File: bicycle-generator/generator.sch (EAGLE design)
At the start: 78 parts, among them IC1 MC34063AD, IC2 MC34063SO, K1 ARK500/2, K2 ARK500/2, K3 ARK500/2, K4 ARK500/2, K5 ARK500/2, K6 HEAT_NPN, K7 ARK500/2, K8 ARK500/2, Q1 IRF3704S, Q2 IRF740, Q3 MPSA56, Q4 IRF740, Q5 MPSA56, T1 BC807, T2 BC807, X1 CV_LED, X2 PWR_LED, X3 5V_SW, X4 5V_LED, X5 5V_OUT

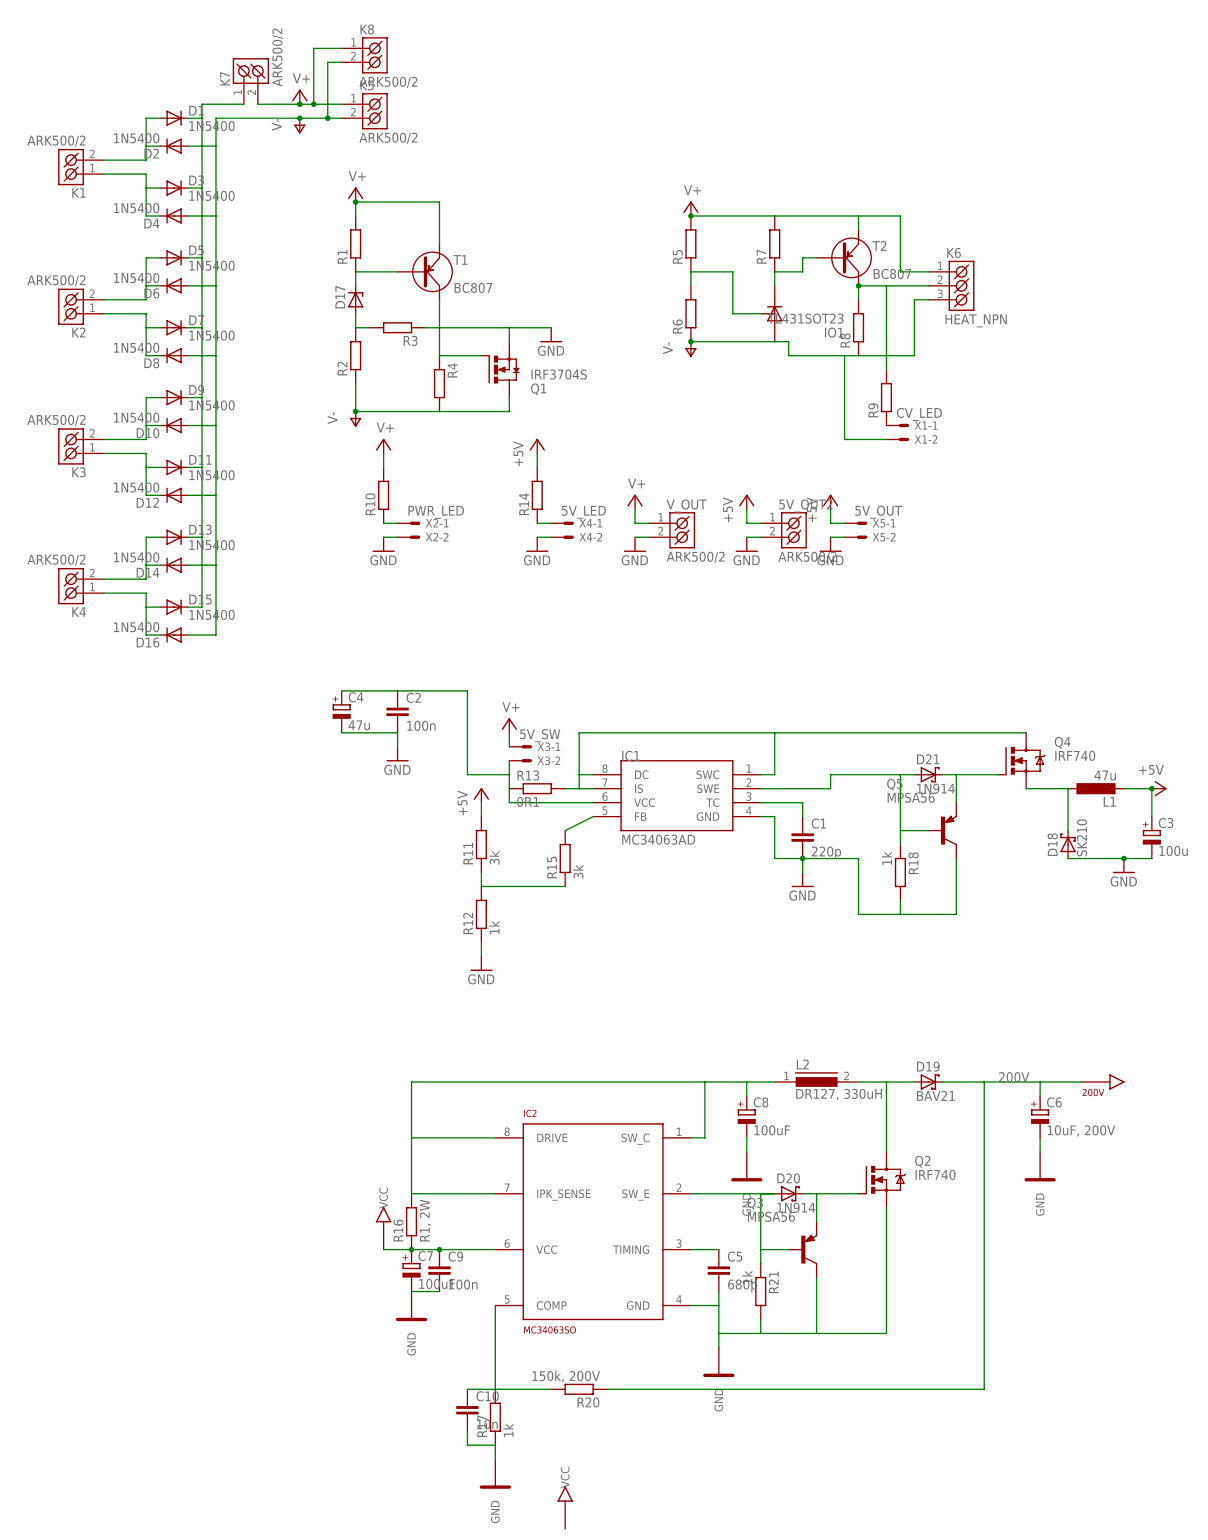
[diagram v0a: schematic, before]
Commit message: First version routed.
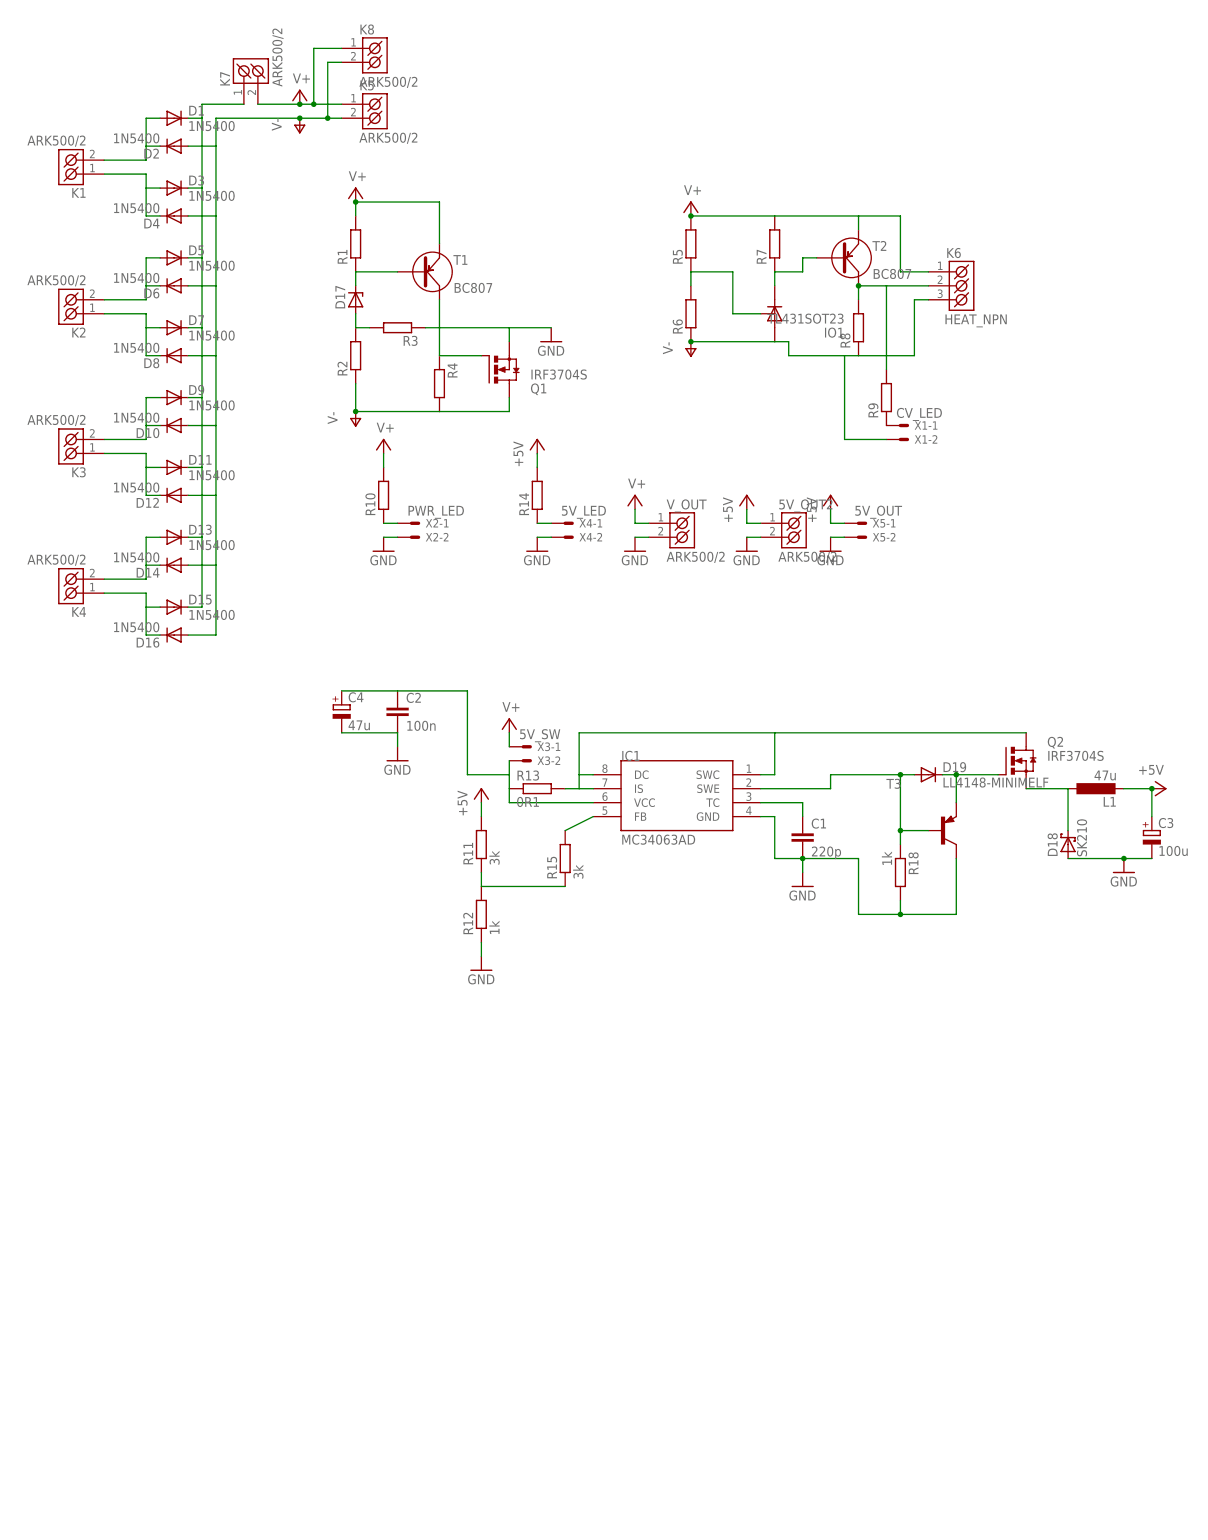
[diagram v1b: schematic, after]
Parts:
- removed C10: 10n, rcl:C-EUC0805
- removed C5: 680p, resistor:C-EUC0805
- removed C6: 10uF, 200V, resistor:CPOL-EUE3.5-10
- removed C7, C8: 100uF, resistor:CPOL-EUD
- removed C9: 100n, rcl:C-EUC0805
- removed D20, D21: 1N914, diode:SCHOTTKY-DIODEDO35-7
- removed IC2: MC34063SO, #Krakonos:MC34063SO
- removed L2: DR127, 330uH, inductors:DR127
- removed Q3, Q5: MPSA56, transistor-pnp:MPSA56
- removed Q4: IRF740, transistor-power:IRF740
- removed R16: R1, 2W, resistor:R-EU_V234/12
- removed R17, R21: 1k, resistor:R-EU_R0805
- removed R20: 150k, 200V, resistor:R-EU_R0805
- added T3: (no value), transistor:BC807-16-PNP-SOT23-BEC
- D19: value BAV21 -> LL4148-MINIMELF; device diode:SCHOTTKY-DIODEDO35-7 -> diode:PMLL41SOD80C
- Q2: value IRF740 -> IRF3704S; device transistor-power:IRF740 -> transistor-power:IRF3704S
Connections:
- removed net 200V: C6.+, D19.C, R20.1
- removed net N$25: C10.1, IC2.COMP, R17.2, R20.2
- removed net N$26: C5.1, IC2.TIMING
- removed net N$29: D19.A, L2.2, Q2.D
- removed net N$30: D20.C, Q2.G, Q3.E
- removed net N$31: D20.A, IC2.SW_E, Q3.B, R21.1
- removed net N$32: C8.+, IC2.DRIVE, IC2.IPK_SENSE, IC2.SW_C, L2.1, R16.2
- removed net N$33: D21.A, IC1.SWE
- removed net VCC: C7.+, C9.1, IC2.VCC, R16.1
- net GND: now also T3.C; no longer C10.2, C5.2, C6.-, C7.-, C8.-, C9.2, IC2.GND, Q2.S, Q3.C, Q5.C, R17.1, R21.2
- net N$15: now also D19.C, Q2.G, T3.E; no longer D21.C, Q4.G, Q5.E
- net N$19: now also Q2.S; no longer Q4.S
- net N$27: now also Q2.D; no longer Q4.D
- net N$28: now also D19.A, IC1.SWE, T3.B; no longer Q5.B

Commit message: Routed board.
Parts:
- L1: device rcl:L-EUPIS2816 -> rcl:L-EUTJ3-U1
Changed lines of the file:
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@@
 <part name="C3" library="rcl" deviceset="CPOL-EU" device="D" value="100u"/>
 <part name="C4" library="rcl" deviceset="CPOL-EU" device="D" value="47u"/>
-<part name="L1" library="rcl" deviceset="L-EU" device="PIS2816" value="47u "/>
+<part name="L1" library="rcl" deviceset="L-EU" device="TJ3-U1" value="47u "/>
 <part name="D18" library="diode" deviceset="SCHOTTKY-DIODE" device="SMD" value="SK210"/>
 <part name="SUPPLY5" library="supply2" deviceset="V+" device=""/>
